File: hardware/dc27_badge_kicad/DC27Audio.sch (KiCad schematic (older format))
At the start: 21 parts, among them U501 CS4344-CZZ, U502 LM4880

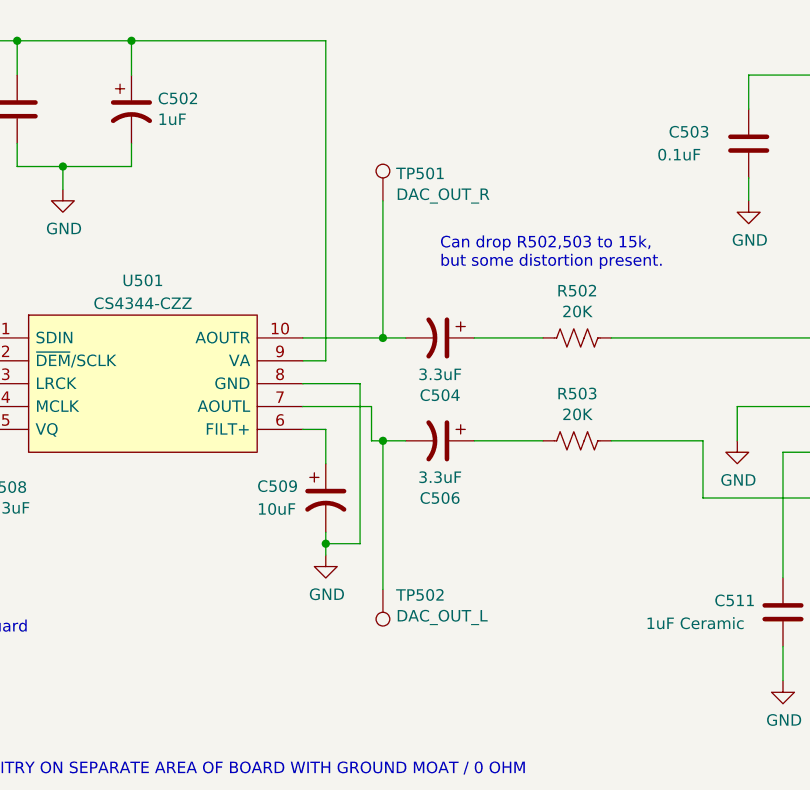
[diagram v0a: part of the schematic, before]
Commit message: check in charging circuit changes
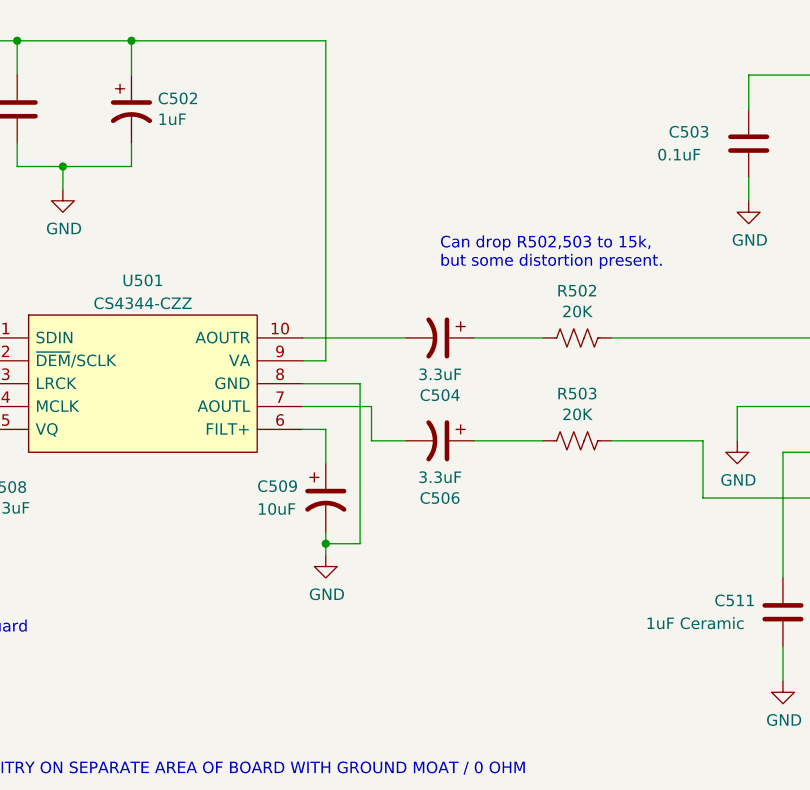
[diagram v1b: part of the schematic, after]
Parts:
- removed TP501: DAC_OUT_R, TestPoint:TestPoint_Pad_D2.0mm, symbol Connector:TestPoint
- removed TP502: DAC_OUT_L, TestPoint:TestPoint_Pad_D2.0mm, symbol Connector:TestPoint
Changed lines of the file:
@@
 	4250 3850 4500 3850
+Wire Wire Line
+	4550 4100 4700 4100
 Wire Wire Line
 	4550 3950 4550 4100
@@
 	5000 4100 5300 4100
 Wire Wire Line
-	4250 3650 4600 3650
+	4250 3650 4700 3650
 Wire Wire Line
 	5000 3650 5300 3650
@@
 Text Notes 4850 3350 0    50   ~ 0
 Can drop R502,503 to 15k, \nbut some distortion present.
-$Comp
-L Connector:TestPoint TP501
-U 1 1 5CE34BE7
-P 4600 3050
-F 0 "TP501" H 4658 3168 50  0000 L CNN
-F 1 "DAC_OUT_R" H 4658 3077 50  0000 L CNN
-F 2 "TestPoint:TestPoint_Pad_D2.0mm" H 4800 3050 50  0001 C CNN
-F 3 "~" H 4800 3050 50  0001 C CNN
-	1    4600 3050
-	1    0    0    -1
-$EndComp
-$Comp
-L Connector:TestPoint TP502
-U 1 1 5CE35CF0
-P 4600 4750
-F 0 "TP502" H 4542 4776 50  0000 R CNN
-F 1 "DAC_OUT_L" H 4542 4867 50  0000 R CNN
-F 2 "TestPoint:TestPoint_Pad_D2.0mm" H 4800 4750 50  0001 C CNN
-F 3 "~" H 4800 4750 50  0001 C CNN
-	1    4600 4750
-	-1   0    0    1
-$EndComp
-Wire Wire Line
-	4600 4750 4600 4100
-Wire Wire Line
-	4550 4100 4600 4100
-Connection ~ 4600 4100
-Wire Wire Line
-	4600 4100 4700 4100
-Wire Wire Line
-	4600 3050 4600 3650
-Connection ~ 4600 3650
-Wire Wire Line
-	4600 3650 4700 3650
 $EndSCHEMATC
